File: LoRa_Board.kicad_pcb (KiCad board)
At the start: 2 copper layers, 68.7 x 25.4 mm, 23 parts, among them J1 USB_C_Receptacle_USB2.0_14P, J2 Conn_Coaxial, U1 ESP32-S3-WROOM-1, U2 AMS1117-3.3, U3 SX1262IMLTRT, Y1 32MHz

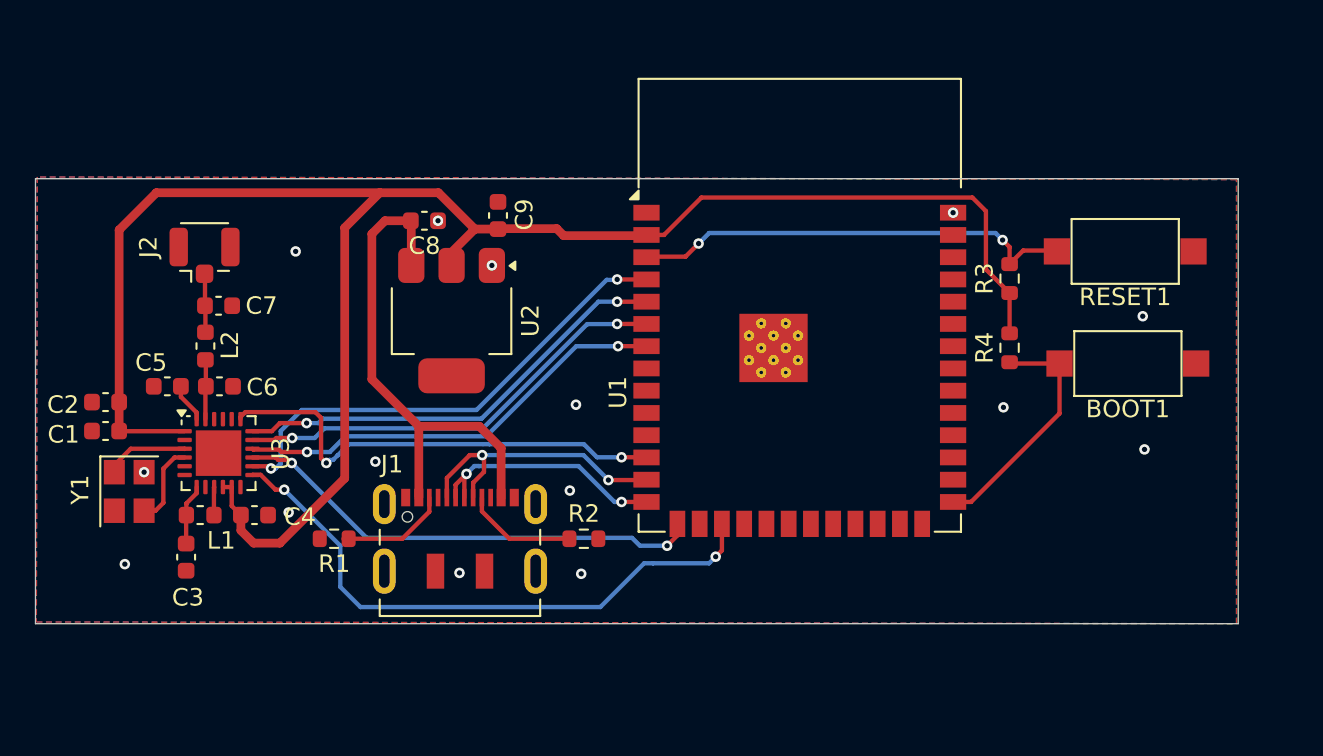
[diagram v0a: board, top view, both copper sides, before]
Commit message: Exported 3d model of CAD + gerbers
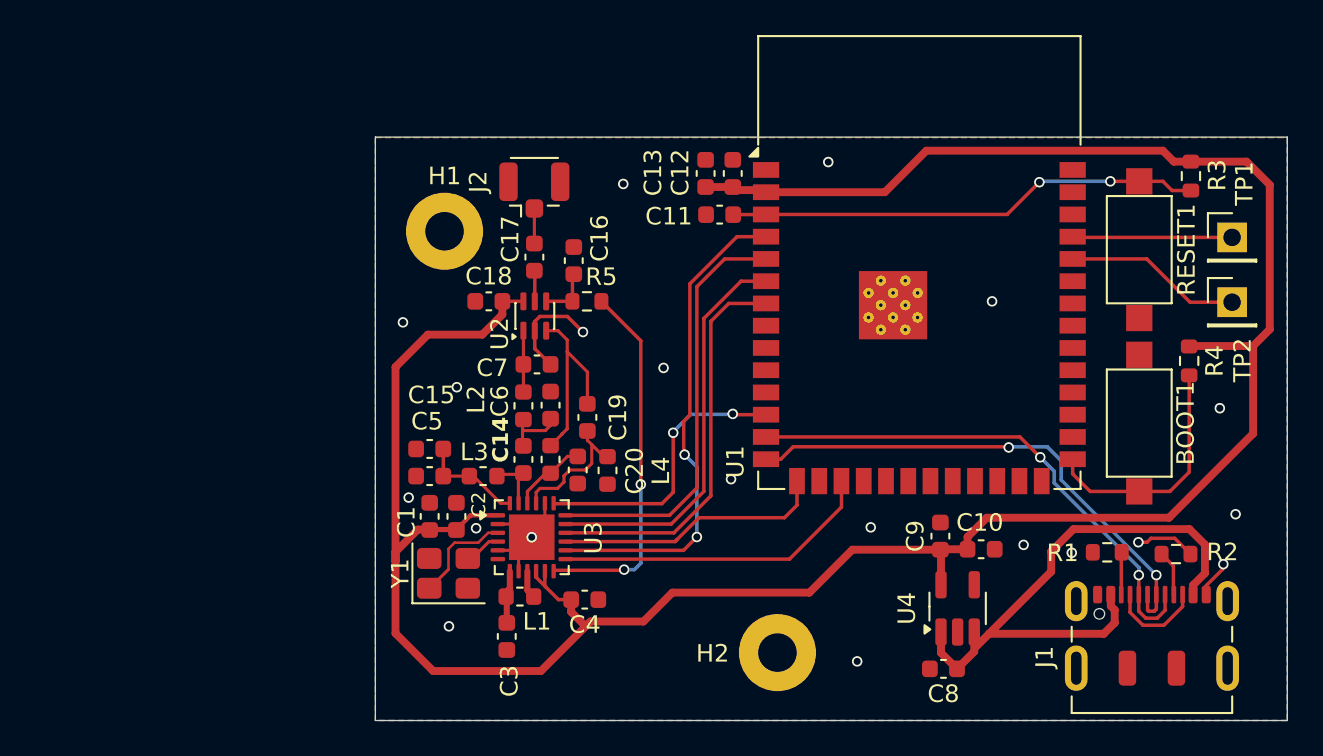
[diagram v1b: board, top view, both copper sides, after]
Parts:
- added C10: 100nF, Capacitor_SMD:C_0603_1608Metric, F.Cu at (137.6, 135.1)
- added C11: 1uF, Capacitor_SMD:C_0603_1608Metric, F.Cu at (122.7, 116.0)
- added C12: 10uF, Capacitor_SMD:C_0603_1608Metric, F.Cu at (123.4, 113.7)
- added C13: 100nF, Capacitor_SMD:C_0603_1608Metric, F.Cu at (121.8, 113.7)
- added C14: 47pF, Capacitor_SMD:C_0603_1608Metric, F.Cu at (111.5, 130.0)
- added C15: 47pF, Capacitor_SMD:C_0603_1608Metric, F.Cu at (106.1, 129.4)
- added C16: 1nF, Capacitor_SMD:C_0603_1608Metric, F.Cu at (114.3, 118.6)
- added C17: 100pF, Capacitor_SMD:C_0603_1608Metric, F.Cu at (112.1, 118.4)
- added C18: 100nF, Capacitor_SMD:C_0603_1608Metric, F.Cu at (109.5, 121.0)
- added C19: 1.8pF, Capacitor_SMD:C_0603_1608Metric, F.Cu at (115.1, 127.6)
- added C20: 2.2pF, Capacitor_SMD:C_0603_1608Metric, F.Cu at (114.5, 130.6)
- added H1: MountingHole, MountingHole:MountingHole_2.2mm_M2_Pad, F.Cu at (107.0, 117.0)
- added H2: MountingHole, MountingHole:MountingHole_2.2mm_M2_Pad, F.Cu at (126.0, 141.0)
- added L3: 47nH, Inductor_SMD:L_0603_1608Metric, F.Cu at (109.2, 130.9)
- added L4: 5,6nH, Inductor_SMD:L_0603_1608Metric, F.Cu at (116.2, 130.6)
- added L5: 6.8nH, Inductor_SMD:L_0603_1608Metric, F.Cu at (113.0, 130.0)
- added R5: R100, Resistor_SMD:R_0603_1608Metric, F.Cu at (115.1, 121.0)
- added TP1: TX0, Connector_PinHeader_2.54mm:PinHeader_1x01_P2.54mm_Vertical, F.Cu at (151.9, 117.3)
- added TP2: RX0, Connector_PinHeader_2.54mm:PinHeader_1x01_P2.54mm_Vertical, F.Cu at (151.9, 121.0)
- added U4: AP2112K-3.3, Package_TO_SOT_SMD:SOT-23-5_HandSoldering, F.Cu at (136.2, 138.5)
- C3: value 100nF -> 470nF
- C8, C9: value 10µF -> 4,7uF
- U2: value AMS1117-3.3 -> PE4259; footprint Package_TO_SOT_SMD:SOT-223-3_TabPin2 -> Package_TO_SOT_SMD:SOT-363_SC-70-6
- moved R1 44.1 mm to (144.8, 135.3)
- moved J1 39.9 mm to (147.3, 140.7)
- moved C8 39.1 mm to (135.4, 141.9)
- moved R2 33.8 mm to (148.7, 135.4)
- moved C9 31.2 mm to (135.2, 134.3)
- moved C2 21.1 mm to (107.6, 133.2), turned to -90 degrees
- moved C4 19.5 mm to (115.0, 138.0)
- moved J2 19.3 mm to (112.1, 114.1)
- moved C1 19.1 mm to (106.1, 133.2), turned to 90 degrees
- moved C6 18.9 mm to (113.0, 126.9), turned to 90 degrees
- moved C3 18.9 mm to (110.5, 140.1)
- moved L1 18.8 mm to (111.2, 137.8)
- moved Y1 18.8 mm to (107.2, 136.5), turned to 0 degrees
- moved U3 18.5 mm to (111.9, 134.4)
- moved C7 18.5 mm to (112.2, 124.5)
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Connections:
- C6 pad 1: Net-(U3-RFO) -> Net-(C14-Pad1)
- C7 pad 1: Net-(J2-In) -> /RF1
- C8 pad 1: GND -> +5V
- C8 pad 2: +5V -> GND
- L2 pad 1: Net-(U3-RFO) -> Net-(C14-Pad1)
- L2 pad 2: Net-(J2-In) -> /RF1
- U1 pad 36: unconnected-(U1-RXD0-Pad36) -> Net-(U1-RXD0)
- U1 pad 37: unconnected-(U1-TXD0-Pad37) -> Net-(U1-TXD0)
- U2 pad 1: GND -> /RF1
- U2 pad 2: +3V3 -> GND
- U2 pad 3: +5V -> Net-(U2-RF2)
- U3 pad 12: unconnected-(U3-DIO2-Pad12) -> /DI12
- U3 pad 21: unconnected-(U3-RFI_P-Pad21) -> /RFI_P
- U3 pad 22: unconnected-(U3-RFI_N-Pad22) -> /RFI_N
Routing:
- net +3V3: track 106.8 -> 147.7 mm
- net /DI12: track 0.00 -> 21.0 mm, vias 0 -> 2
- net GND: track 0.00 -> 19.6 mm, vias 15 -> 20
- net /DIO1: track 34.2 -> 18.5 mm, vias 2 -> 0
- net /USB_D+: track 14.3 -> 29.7 mm
- net /USB_D-: track 16.4 -> 30.0 mm
- net /RESET: track 27.2 -> 15.4 mm, vias 2 -> 0
- net Net-(U2-RF2): track 0.00 -> 11.3 mm
- net /NSS: track 26.7 -> 16.3 mm
- net Net-(U1-RXD0): track 0.00 -> 10.1 mm
- net Net-(U1-TXD0): track 0.00 -> 9.12 mm
- net /RFI_P: track 0.00 -> 8.19 mm
- net (no net): track 0.00 -> 5.45 mm
- net +5V: track 29.3 -> 34.5 mm
- net /RFI_N: track 0.00 -> 4.38 mm
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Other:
- board size 68.7 x 25.4 mm -> 52.1 x 33.3 mm
